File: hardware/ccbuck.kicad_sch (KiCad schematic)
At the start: 37 parts, among them J4 PWM/PFM, Q11 2N7002, U1 TPS552872RYQR

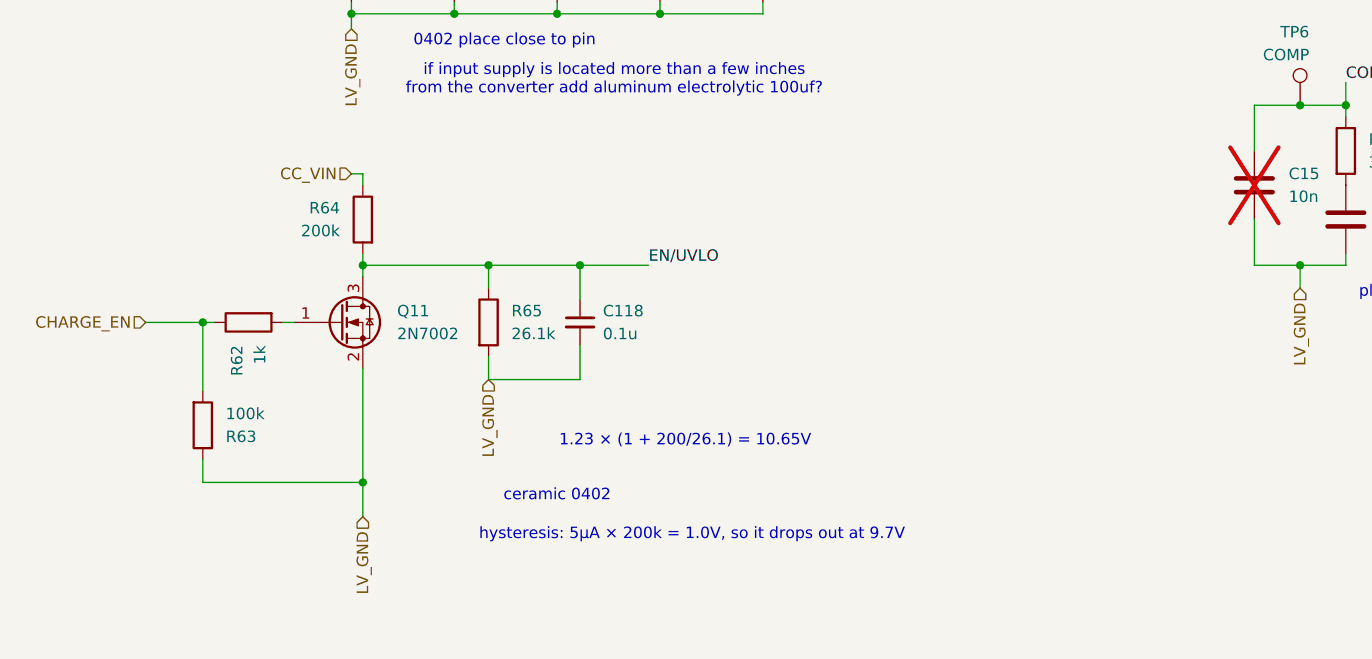
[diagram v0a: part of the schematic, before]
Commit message: oops
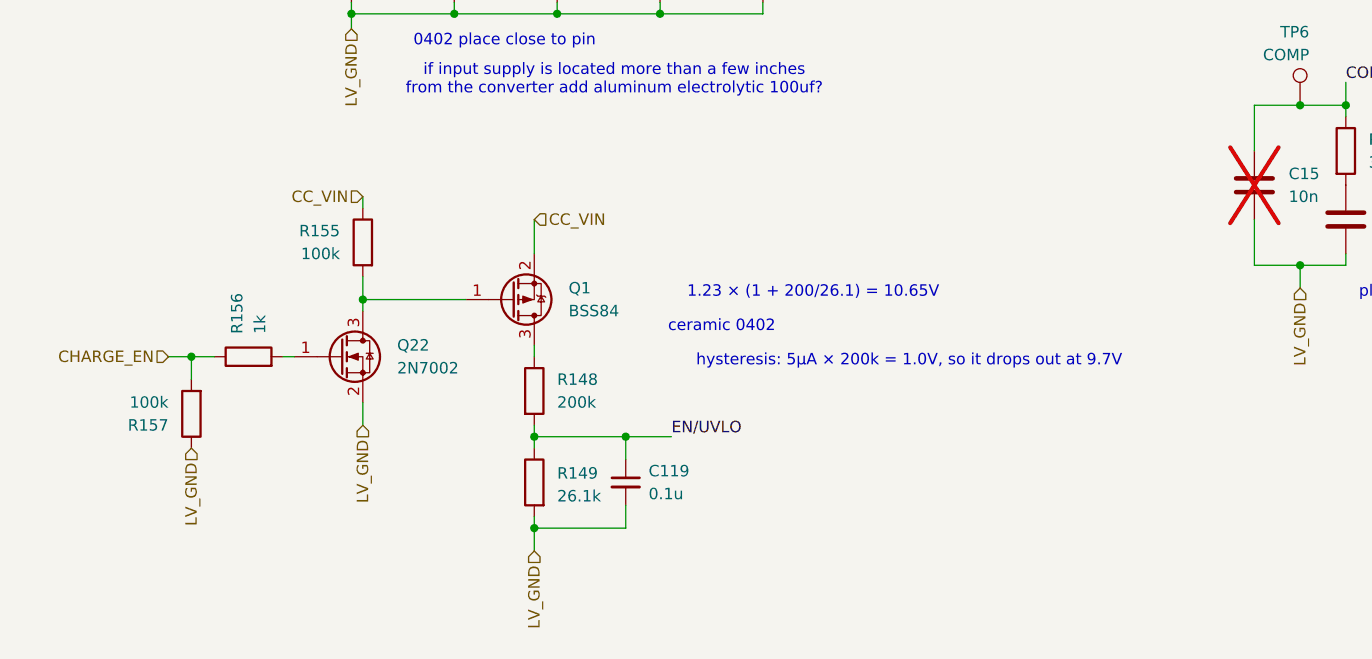
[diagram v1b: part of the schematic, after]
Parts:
- removed C118: 0.1u, Capacitor_SMD:C_0402_1005Metric_Pad0.74x0.62mm_HandSolder, symbol Device:C_Small
- removed Q11: 2N7002, Package_TO_SOT_SMD:SOT-23, symbol Transistor_FET:2N7002
- removed R62: 1k, Resistor_SMD:R_0603_1608Metric_Pad0.98x0.95mm_HandSolder, symbol Device:R
- removed R63: 100k, Resistor_SMD:R_0603_1608Metric_Pad0.98x0.95mm_HandSolder, symbol Device:R
- removed R64: 200k, Resistor_SMD:R_0603_1608Metric_Pad0.98x0.95mm_HandSolder, symbol Device:R
- removed R65: 26.1k, Resistor_SMD:R_0603_1608Metric_Pad0.98x0.95mm_HandSolder, symbol Device:R
- added C119: 0.1u, Capacitor_SMD:C_0603_1608Metric_Pad1.08x0.95mm_HandSolder, symbol Device:C_Small
- added Q1: BSS84, Package_TO_SOT_SMD:SOT-23, symbol Transistor_FET:BSS84
- added Q22: 2N7002, Package_TO_SOT_SMD:SOT-23, symbol Transistor_FET:2N7002
- added R148: 200k, Resistor_SMD:R_0603_1608Metric_Pad0.98x0.95mm_HandSolder, symbol Device:R
- added R149: 26.1k, Resistor_SMD:R_0603_1608Metric_Pad0.98x0.95mm_HandSolder, symbol Device:R
- added R155, R157: 100k, Resistor_SMD:R_0603_1608Metric_Pad0.98x0.95mm_HandSolder, symbol Device:R
- added R156: 1k, Resistor_SMD:R_0603_1608Metric_Pad0.98x0.95mm_HandSolder, symbol Device:R
- C10, C11, C12, C13, C20, C21, C22, C23: P/N (none) -> MLASU168SB5105KTNA01
- C14: footprint Capacitor_SMD:C_0402_1005Metric_Pad0.74x0.62mm_HandSolder -> Capacitor_SMD:C_0603_1608Metric_Pad1.08x0.95mm_HandSolder; LCSC P/N (none) -> C14663; P/N (none) -> MLASH168SB7104KTNA01
- C15: LCSC P/N (none) -> C57112; P/N (none) -> MSASH168SB5103KTNA01
- C16: P/N (none) -> 06035C472K4T2A
- C17: LCSC P/N C22387800 -> C6962403; P/N (none) -> 08055D475KAT4A
- C18, C19: P/N (none) -> MLASH168SB7104KTNA01
- U1: LCSC P/N (none) -> C22427496; P/N (none) -> TPS552872RYQR
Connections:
- net CC_VIN: now also Q1.2 (S), R155.1
- net CHARGE_EN: now also R156.1, R157.2
- net EN/UVLO: now also C119.1, R148.2, R149.1
- net LV_GND: now also C119.2, Q22.2 (S), R149.2, R157.1
- new net: Q1.1 (G), Q22.3 (D), R155.2
- new net: Q1.3 (D), R148.1
- new net: Q22.1 (G), R156.2

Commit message: added most p/n, still in progress but saving
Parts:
- D8, D9: LCSC P/N (none) -> -- mixed values --; P/N (none) -> -- mixed values --
- R148: P/N (none) -> 0603WAF2003T5E
- R155: Assemble (none) -> -- mixed values --; LCSC P/N C25811 -> C25803; P/N (none) -> CRCW0603100KFKEE
- R156: Assemble (none) -> -- mixed values --; LCSC P/N (none) -> C21190; P/N (none) -> CRCW06031K00FKEI
- R157, R23, R24, R29: Assemble (none) -> -- mixed values --; LCSC P/N (none) -> C25803; P/N (none) -> CRCW0603100KFKEE
- R20: LCSC P/N (none) -> C177599; P/N (none) -> RCT0349K9FLF
- R25: LCSC P/N (none) -> C177300; P/N (none) -> RCT0330KJLF
- R26, R27: LCSC P/N (none) -> C177867; P/N (none) -> RCT031K3FLF
- R30: LCSC P/N (none) -> C177496; P/N (none) -> RCT038K66FLF
